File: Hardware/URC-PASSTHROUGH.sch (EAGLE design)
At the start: 7 parts, among them J1 RJ45-X1-METAL, J2 RJ45-X1-METAL

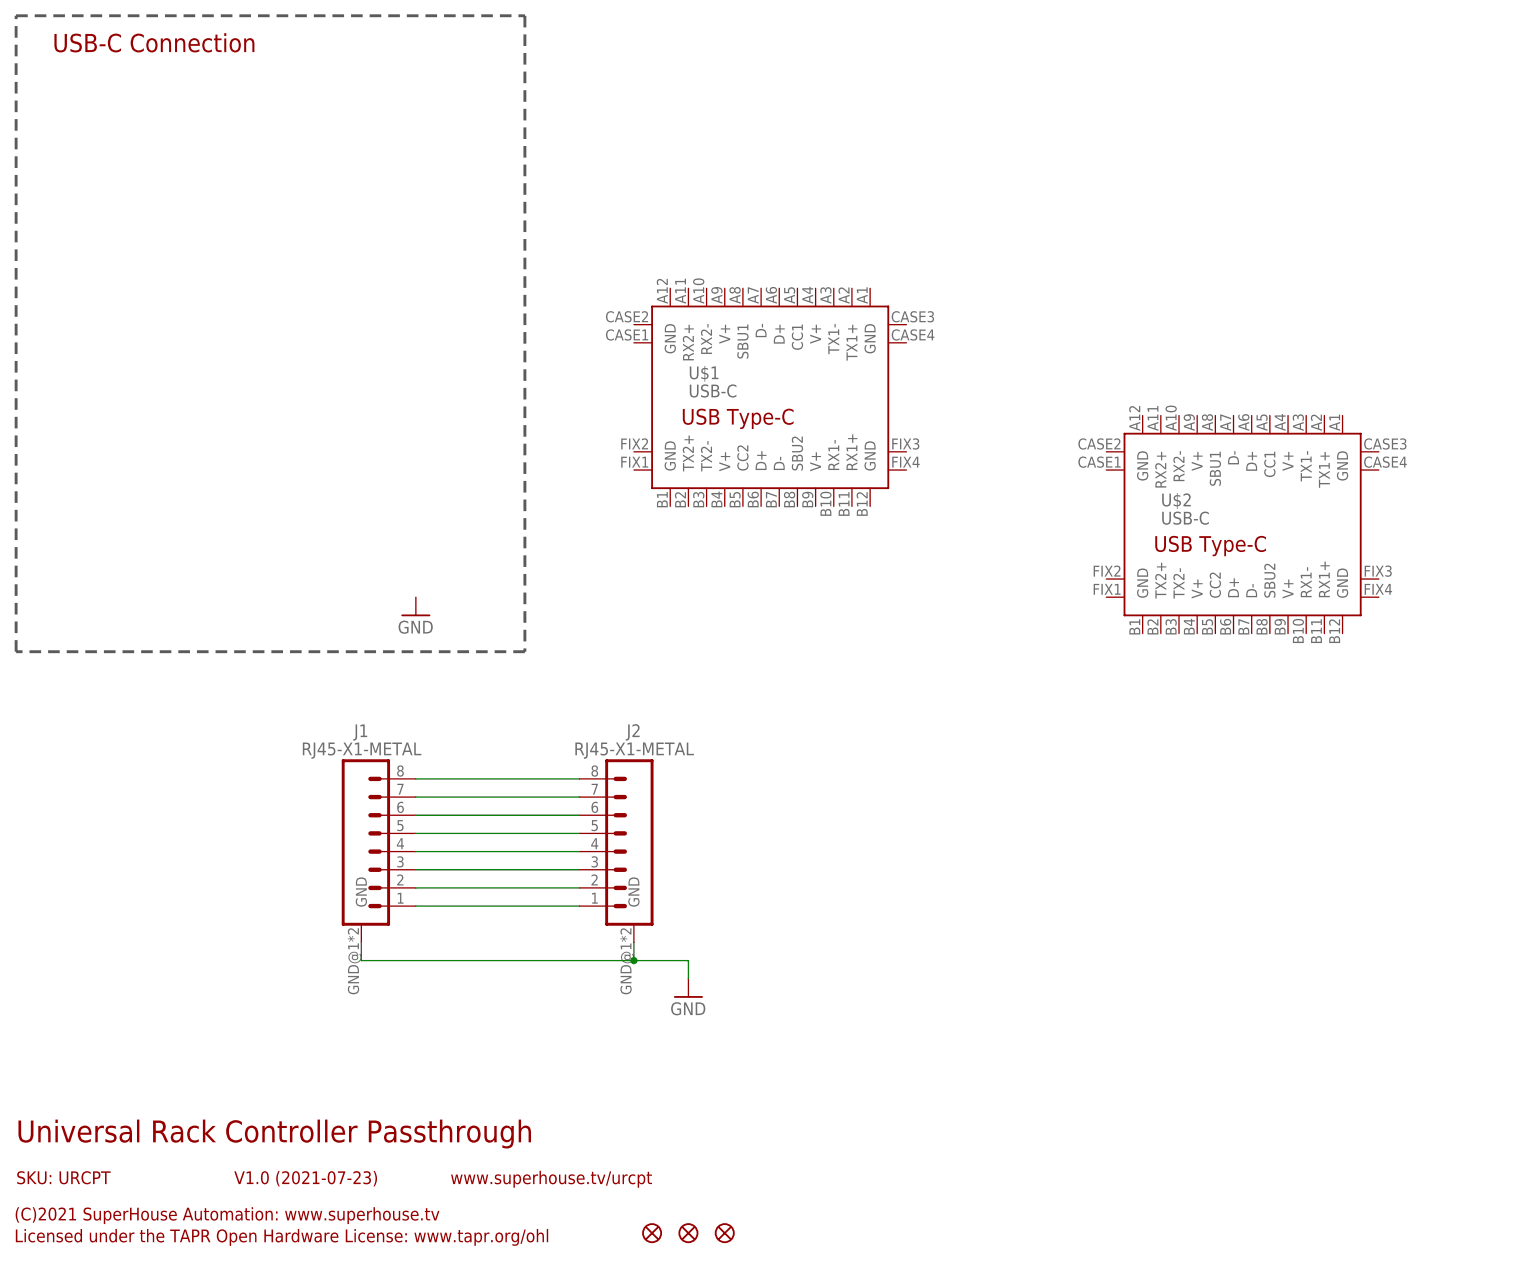
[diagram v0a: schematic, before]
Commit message: Schematic progress for passthrough edition.
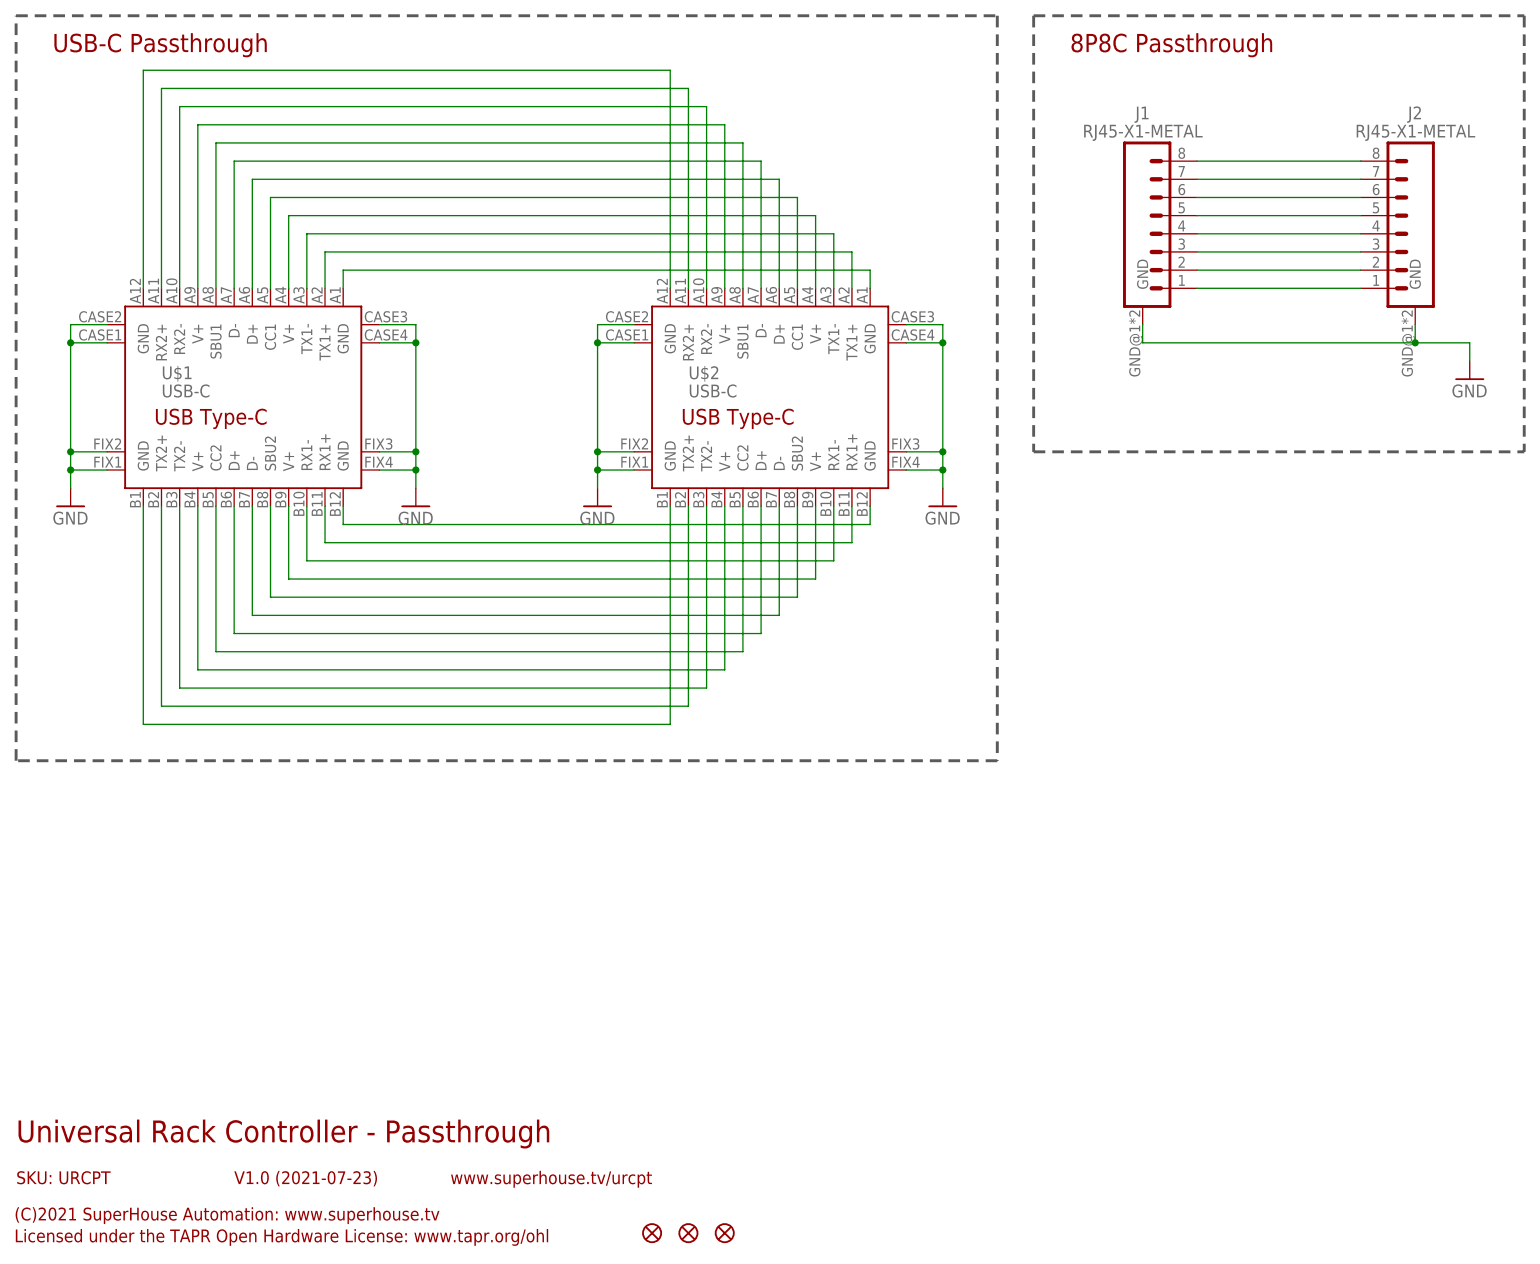
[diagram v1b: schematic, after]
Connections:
- new net N$10: U$1.TX1+, U$2.TX1+
- new net N$11: U$1.TX1-, U$2.TX1-
- new net N$12: U$1.V+@A4, U$2.V+@A4
- new net N$13: U$1.CC1, U$2.CC1
- new net N$14: U$1.D+@A6, U$2.D+@A6
- new net N$15: U$1.D-@A7, U$2.D-@A7
- new net N$16: U$1.SBU1, U$2.SBU1
- new net N$17: U$1.V+@A9, U$2.V+@A9
- new net N$18: U$1.RX2-, U$2.RX2-
- new net N$19: U$1.RX2+, U$2.RX2+
- new net N$20: U$1.GND@A12, U$2.GND@A12
- new net N$21: U$1.GND@B12, U$2.GND@B12
- new net N$22: U$1.RX1+, U$2.RX1+
- new net N$23: U$1.RX1-, U$2.RX1-
- new net N$24: U$1.V+@B9, U$2.V+@B9
- new net N$25: U$1.SBU2, U$2.SBU2
- new net N$26: U$1.D-@B7, U$2.D-@B7
- new net N$27: U$1.D+@B6, U$2.D+@B6
- new net N$28: U$1.CC2, U$2.CC2
- new net N$29: U$1.V+@B4, U$2.V+@B4
- new net N$30: U$1.TX2-, U$2.TX2-
- new net N$31: U$1.TX2+, U$2.TX2+
- new net N$32: U$1.GND@B1, U$2.GND@B1
- new net N$9: U$1.GND@A1, U$2.GND@A1
- net GND: now also U$1.GND@CASE1, U$1.GND@CASE2, U$1.GND@CASE3, U$1.GND@CASE4, U$1.GND@FIX1, U$1.GND@FIX2, U$1.GND@FIX3, U$1.GND@FIX4, U$2.GND@CASE1, U$2.GND@CASE2, U$2.GND@CASE3, U$2.GND@CASE4, U$2.GND@FIX1, U$2.GND@FIX2, U$2.GND@FIX3, U$2.GND@FIX4
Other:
- note added: "8P8C Passthrough"
- note added: "USB-C Passthrough"
- note added: "Universal Rack Controller - Passthrough"
- note removed: "USB-C Connection"
- note removed: "Universal Rack Controller Passthrough"
- moved on the sheet: J1, J2, U$1, U$2
